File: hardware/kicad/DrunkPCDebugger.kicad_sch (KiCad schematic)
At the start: 96 parts, among them Q1 2N7002K-T1-GE3, Q2 AO3401A, Q3 AO3401A, SW2 TS3643TP, SW3 TS3643TP, U1 74LVX4245MTCX, U10 A-SC6302R6AGHC-A03-2T, U2 STM32H723VGT6, U3 74LVX4245MTCX, U4 74LVX4245MTCX, U5 X6521FV-2X27-C85D32, U6 AMS1117-3_3, U7 74LVX4245MTCX, U8 SN74LVC3G17DCTR, U9 SN74AHCT125DR, X1 X322525MOB4SI

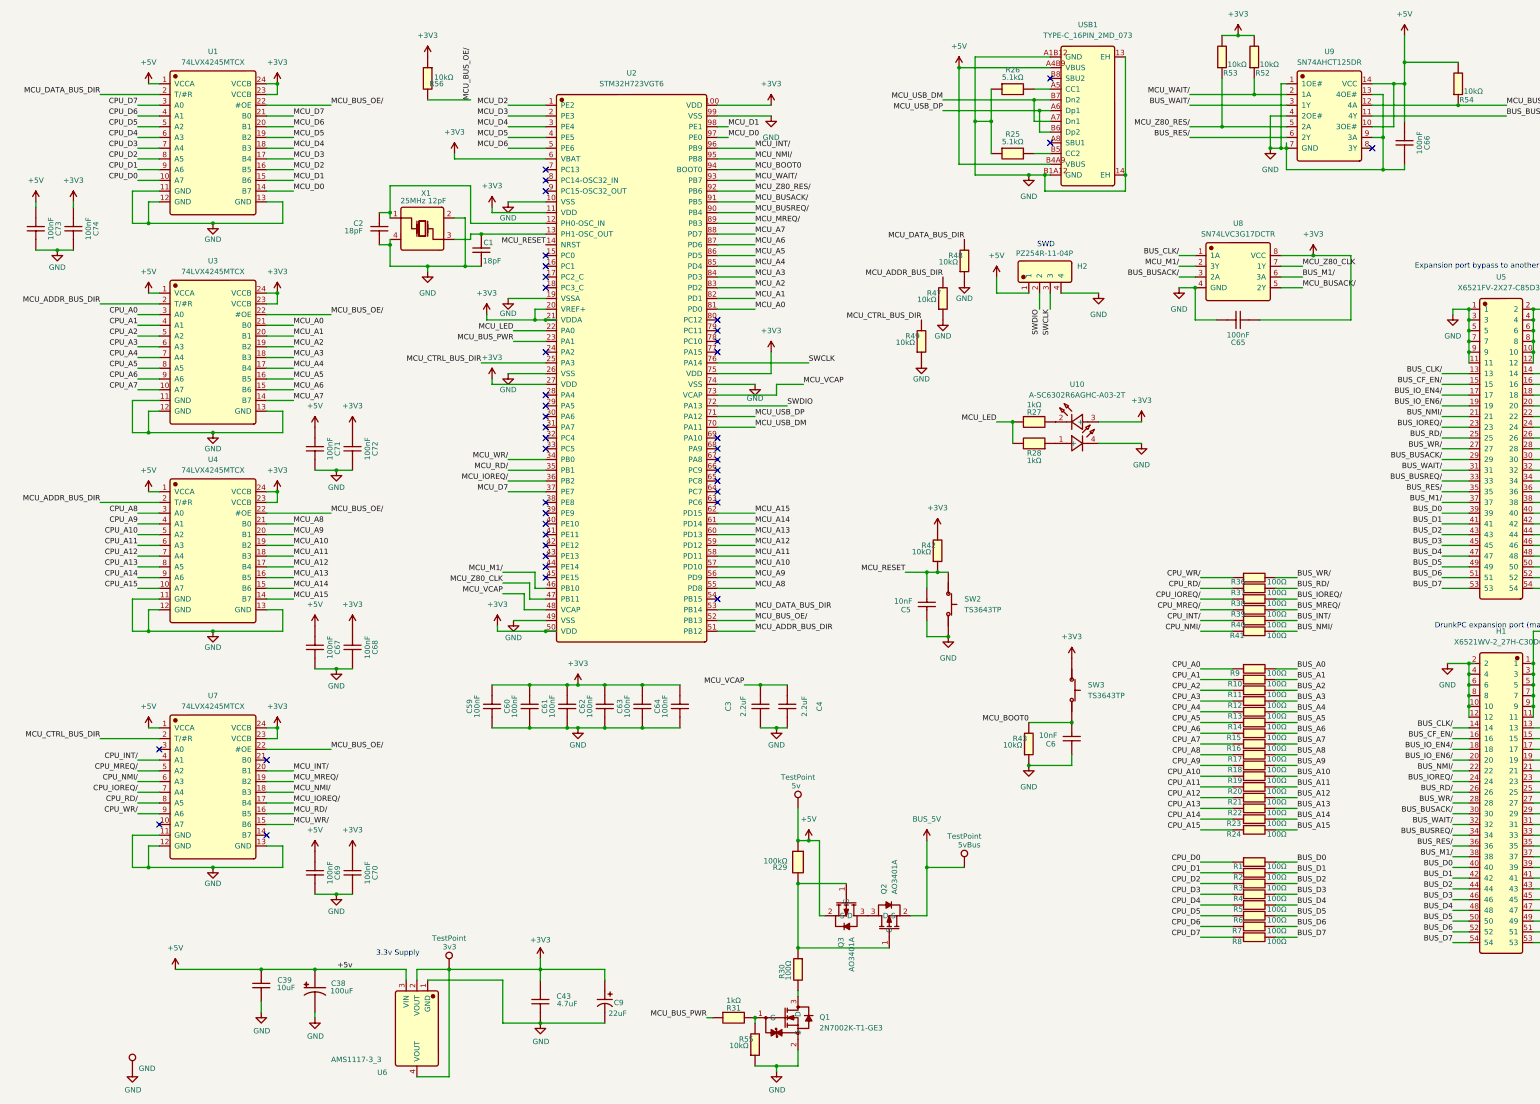
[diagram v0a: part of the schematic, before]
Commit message: Replace components
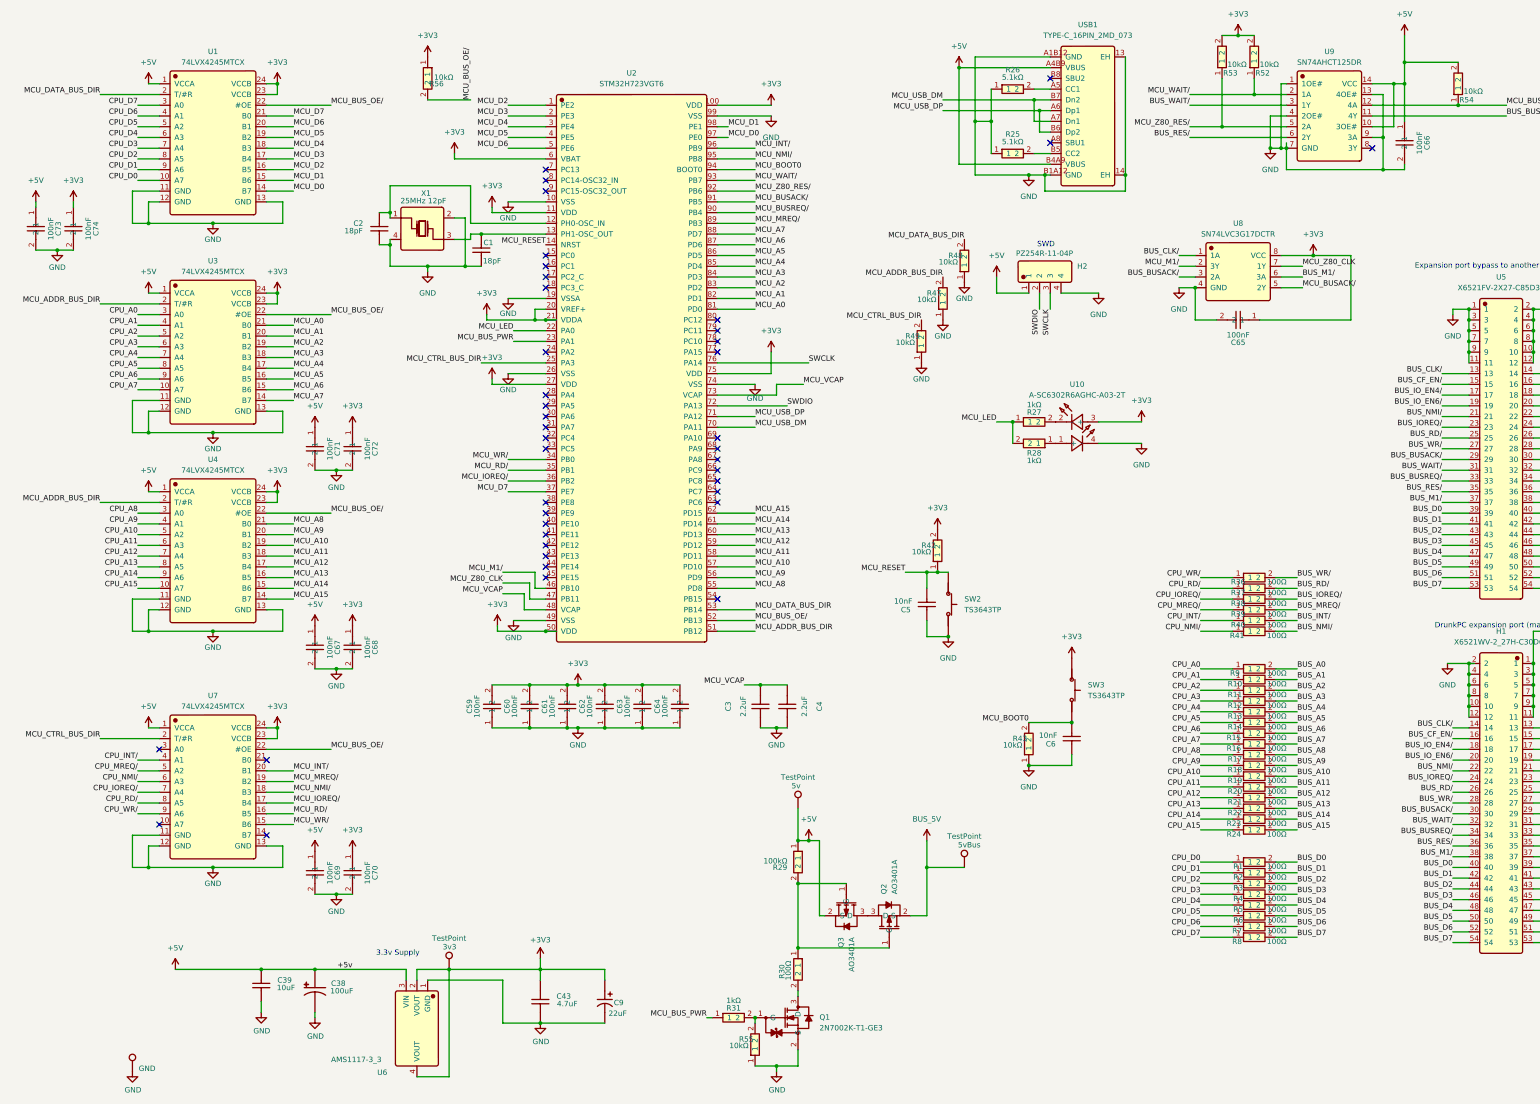
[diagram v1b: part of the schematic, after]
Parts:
- C59, C60, C61, C62, C63, C64, C65, C66, C67, C68, C69, C70, C71, C72, C73, C74: value CL10B104KB8NNNC -> CC0603KRX7R9BB104; symbol JLCImport:CL10B104KB8NNNC -> JLCImport:CC0603KRX7R9BB104; LCSC C1591 -> C14663; Manufacturer Samsung Electro-Mechanics -> YAGEO; Manufacturer Part CL10B104KB8NNNC -> CC0603KRX7R9BB104
- R1, R10, R11, R12, R13, R14, R15, R16, R17, R18, R19, R2, R20, R21, R22, R23, R24, R3, R30, R36, R37, R38, R39, R4, R40, R41, R5, R6, R7, R8, R9: value RT0603BRD07100RL -> 0603WAF1000T5E; symbol JLCImport:RT0603BRD07100RL -> JLCImport:0603WAF1000T5E; LCSC C122970 -> C22775; Manufacturer YAGEO -> UNI-ROYAL(Uniroyal Elec); Manufacturer Part RT0603BRD07100RL -> 0603WAF1000T5E
- R25, R26: value FRC0603F5101TS -> 0603WAF5101T5E; symbol JLCImport:FRC0603F5101TS -> JLCImport:0603WAF5101T5E; LCSC C2907044 -> C23186; Manufacturer FOJAN -> UNI-ROYAL(Uniroyal Elec); Manufacturer Part FRC0603F5101TS -> 0603WAF5101T5E
- R27, R28, R31: value FRC0603F1001TS -> 0603WAF1001T5E; symbol JLCImport:FRC0603F1001TS -> JLCImport:0603WAF1001T5E; LCSC C2907002 -> C21190; Manufacturer FOJAN -> UNI-ROYAL(Uniroyal Elec); Manufacturer Part FRC0603F1001TS -> 0603WAF1001T5E
- R29: value FRC0603J104_TS -> 0603WAF1003T5E; symbol JLCImport:FRC0603J104_TS -> JLCImport:0603WAF1003T5E; LCSC C2907088 -> C25803; Manufacturer FOJAN -> UNI-ROYAL(Uniroyal Elec); Manufacturer Part FRC0603J104 TS -> 0603WAF1003T5E
- R42, R43, R47, R48, R49, R52, R53, R54, R55, R56: value RT0603BRD0710KL -> 0603WAF1002T5E; symbol JLCImport:RT0603BRD0710KL -> JLCImport:0603WAF1002T5E; LCSC C95204 -> C25804; Manufacturer YAGEO -> UNI-ROYAL(Uniroyal Elec); Manufacturer Part RT0603BRD0710KL -> 0603WAF1002T5E

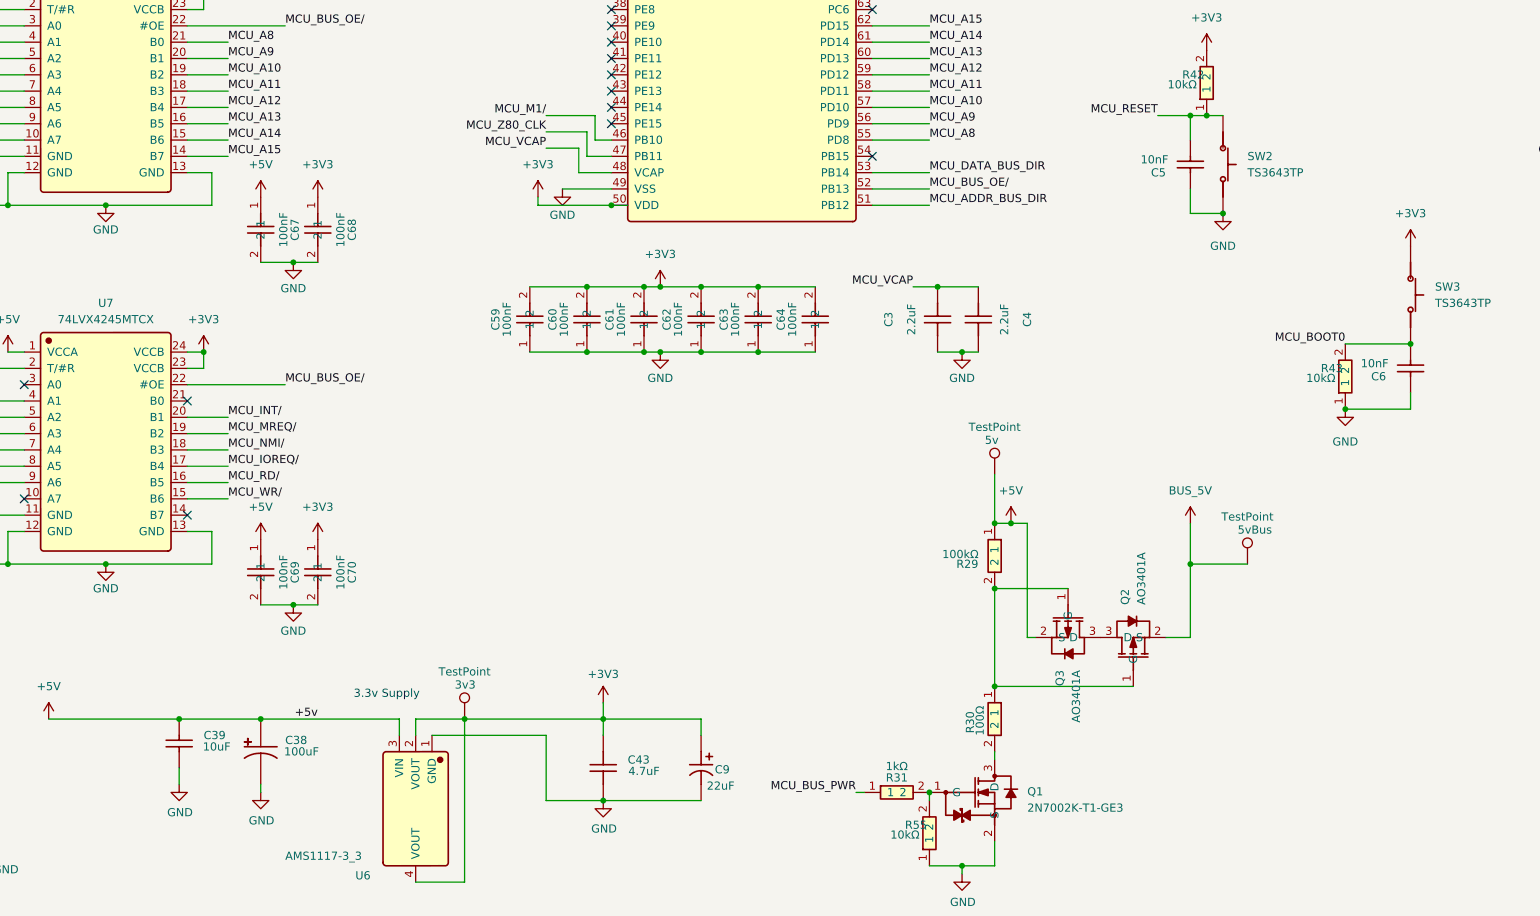
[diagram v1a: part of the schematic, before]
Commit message: Replace parts
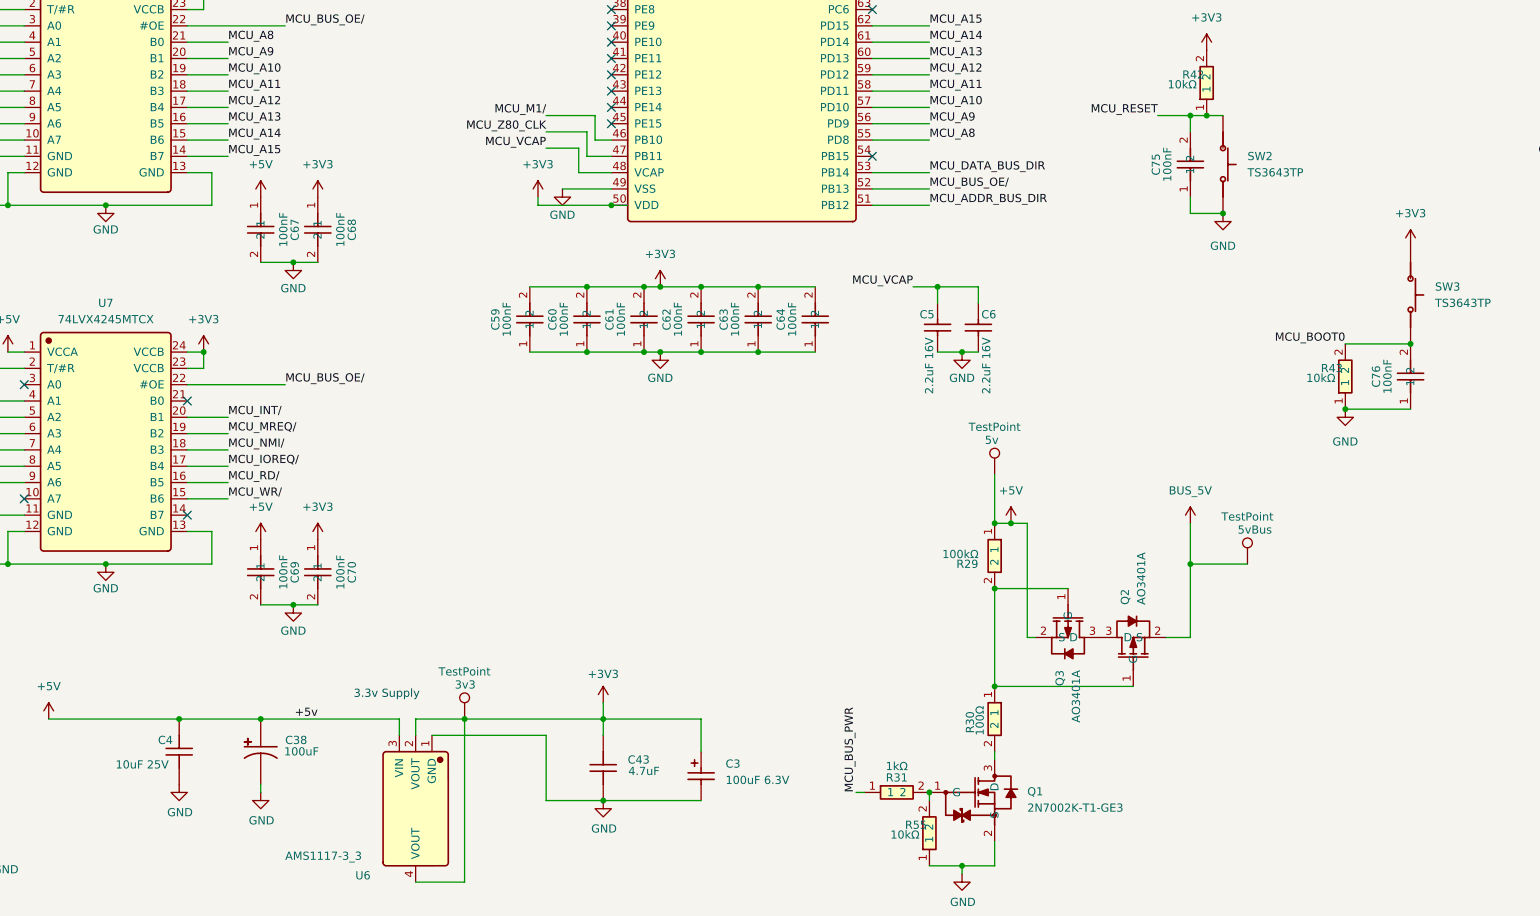
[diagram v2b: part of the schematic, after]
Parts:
- removed C3, C4: GRM21BR71A225KA01L, Capacitor_SMD:C_0805_2012Metric, symbol JLCImport:GRM21BR71A225KA01L
- removed C39: GCM21BR71A106KE22L, JLCImport:GCM21BR71A106KE22L, symbol JLCImport:GCM21BR71A106KE22L
- removed C5, C6: CC0603KRX7R0BB103, Capacitor_SMD:C_0603_1608Metric, symbol JLCImport:CC0603KRX7R0BB103
- removed C9: 25TQC22MYFB, JLCImport:25TQC22MYFB, symbol JLCImport:25TQC22MYFB
- added C3: 100uF 6.3V, Capacitor_Tantalum_SMD:CP_EIA-3528-21_Kemet-B, symbol JLCImport:TAJB107K006RNJ
- added C4: 10uF 25V, Capacitor_SMD:C_0805_2012Metric, symbol JLCImport:CL21A106KAYNNNE
- added C5, C6: 2.2uF 16V, Capacitor_SMD:C_0603_1608Metric, symbol JLCImport:CL10A225KO8NNNC
- added C75, C76: CC0603KRX7R9BB104, Capacitor_SMD:C_0603_1608Metric, symbol JLCImport:CC0603KRX7R9BB104
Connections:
- net +3V3: now also C3.1
- net +5V: now also C4.1
- net GND: now also C3.2, C4.2, C5.2, C6.2, C75.1, C76.1
- net MCU_BOOT0: now also C76.2
- net MCU_RESET: now also C75.2
- net MCU_VCAP: now also C5.1, C6.1
